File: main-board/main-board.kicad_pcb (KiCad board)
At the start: 2 copper layers, 93 x 46.5 mm, 21 parts, among them J1 AC_IN, J2 AC_OUT, J3 AC_OUT, K1 SRD-05VDC-SL-C, Q1 MMBT2222ALT1G, Q2 BTA12-600B, U1 LTV-354T, U2 Arduino-nano-BLE-33, U3 FODM3022, U4 SCD40-D-R2, U5 SGP40-D-R4

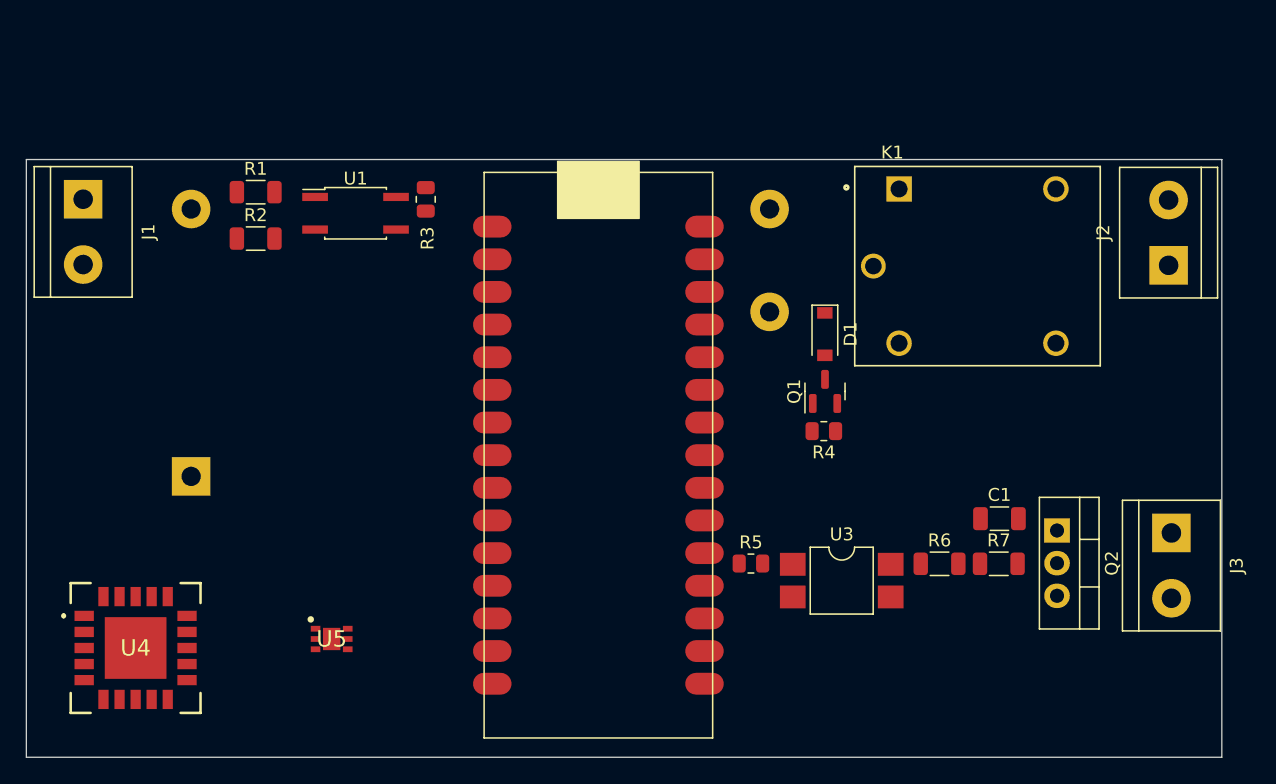
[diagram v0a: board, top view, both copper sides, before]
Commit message: update main board
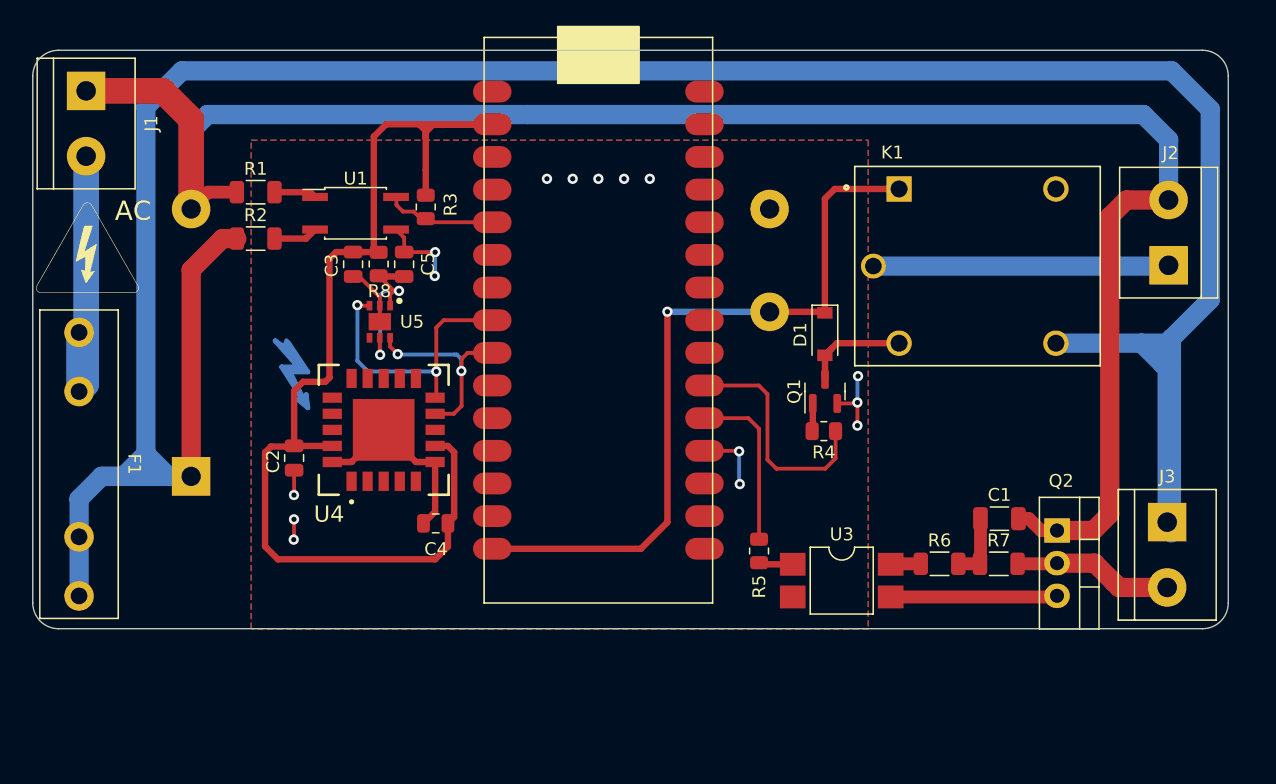
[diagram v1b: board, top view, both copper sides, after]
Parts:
- added C2: 10uF, Capacitor_SMD:C_0805_2012Metric, F.Cu at (88.3, 72.7)
- added C3: 10uF, Capacitor_SMD:C_0805_2012Metric, F.Cu at (92.9, 57.6)
- added C4: 10uF, Capacitor_SMD:C_0805_2012Metric, F.Cu at (99.3, 77.8)
- added C5: 1uF, Capacitor_SMD:C_0805_2012Metric, F.Cu at (96.9, 57.6)
- added F1: Fuse, Fuse:Fuseholder_Littelfuse_100_series_5x20mm, F.Cu at (71.6, 63.0)
- added G***: LOGO, high_voltage, F.Cu at (72.2, 56.4)
- added R8: 4.7R, Resistor_SMD:R_0805_2012Metric, F.Cu at (94.9, 57.6)
- added REF**: Symbol_Highvoltage_Type2_CopperTop_Small, Symbol:Symbol_Highvoltage_Type2_CopperTop_Small, B.Cu at (88.0, 66.9)
- moved U4 25.7 mm to (95.3, 70.5), turned to 90 degrees
- moved U5 25.0 mm to (95.0, 62.1), turned to -90 degrees
- moved U2 10.5 mm to (112.0, 62.0)
- moved J1 8.43 mm to (72.2, 44.2)
- moved R5 1.17 mm to (124.5, 80.0), turned to -90 degrees
- moved J3 0.90 mm to (156.2, 77.7)
- moved R3 0.59 mm to (98.6, 53.2)
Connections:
- J1 pad 2: LINE -> Net-(F1-Pad1)
- PS1 pad 1: Net-(F1-Pad2) -> LINE
- R1 pad 1: LINE -> NEUT
- R2 pad 1: NEUT -> LINE
- U2 pad 20: unconnected-(U2-Pad20) -> /ControlSignal2
- U2 pad 21: unconnected-(U2-Pad21) -> /ControlSignal1
- U2 pad 5: unconnected-(U2-Pad5) -> /ZeroDetector
- U4 pad 10: (no net) -> /SDA
- U4 pad 19: unconnected-(U4-Pad19) -> +3V3
- U4 pad 20: Net-(U4-Pad20) -> GND
- U4 pad 21: Net-(U4-Pad20) -> GND
- U4 pad 6: Net-(U4-Pad20) -> GND
- U4 pad 7: unconnected-(U4-Pad7) -> +3V3
- U4 pad 9: unconnected-(U4-Pad9) -> /SCL
- U5 pad 1: unconnected-(U5-Pad1) -> Net-(C5-Pad1)
- U5 pad 2: unconnected-(U5-Pad2) -> GND
- U5 pad 3: unconnected-(U5-Pad3) -> /SDA
- U5 pad 4: unconnected-(U5-Pad4) -> GND
- U5 pad 5: unconnected-(U5-Pad5) -> Net-(C5-Pad1)
- U5 pad 6: unconnected-(U5-Pad6) -> /SCL
- U5 pad 7: unconnected-(U5-Pad7) -> GND
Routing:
- net LINE: track 0.00 -> 223.8 mm
- net NEUT: track 0.00 -> 144.6 mm
- net +3V3: track 0.00 -> 88.2 mm
- net +5V: track 0.00 -> 58.1 mm, vias 0 -> 1
- net GND: track 0.00 -> 40.4 mm, vias 0 -> 15
- net Net-(F1-Pad1): track 0.00 -> 23.1 mm
- net Net-(J2-Pad1): track 0.00 -> 23.0 mm
- net /SDA: track 0.00 -> 21.9 mm, vias 0 -> 2
- net /ControlSignal1: track 0.00 -> 18.3 mm
- net /SCL: track 0.00 -> 16.1 mm, vias 0 -> 2
- net Net-(C5-Pad1): track 0.00 -> 14.4 mm, vias 0 -> 2
- net /ControlSignal2: track 0.00 -> 13.2 mm
- net Net-(Q2-Pad3): track 0.00 -> 13.0 mm
- net Net-(J3-Pad2): track 0.00 -> 12.4 mm
- net Net-(D1-Pad2): track 0.00 -> 10.6 mm
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- added copper zone on B.Cu, net GND
- added copper zone on F.Cu, net GND
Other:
- board size 93 x 46.5 mm -> 93 x 45 mm
- board text added: "AC"
